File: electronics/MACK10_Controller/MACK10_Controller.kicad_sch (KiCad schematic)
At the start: 31 parts, among them J1 Stepper Motor, J10 I/O, J3 Load Cell, J4 24V IN, J5 SSD1306, J6 INPUT, J7 E_STOP, J8 LIM_TOP, J9 LIM_BOT, U1 U1 ESP32_DEVKIT_30P, U2 HX711, U3 TMC2208, U4 LM2596 Buck Converter

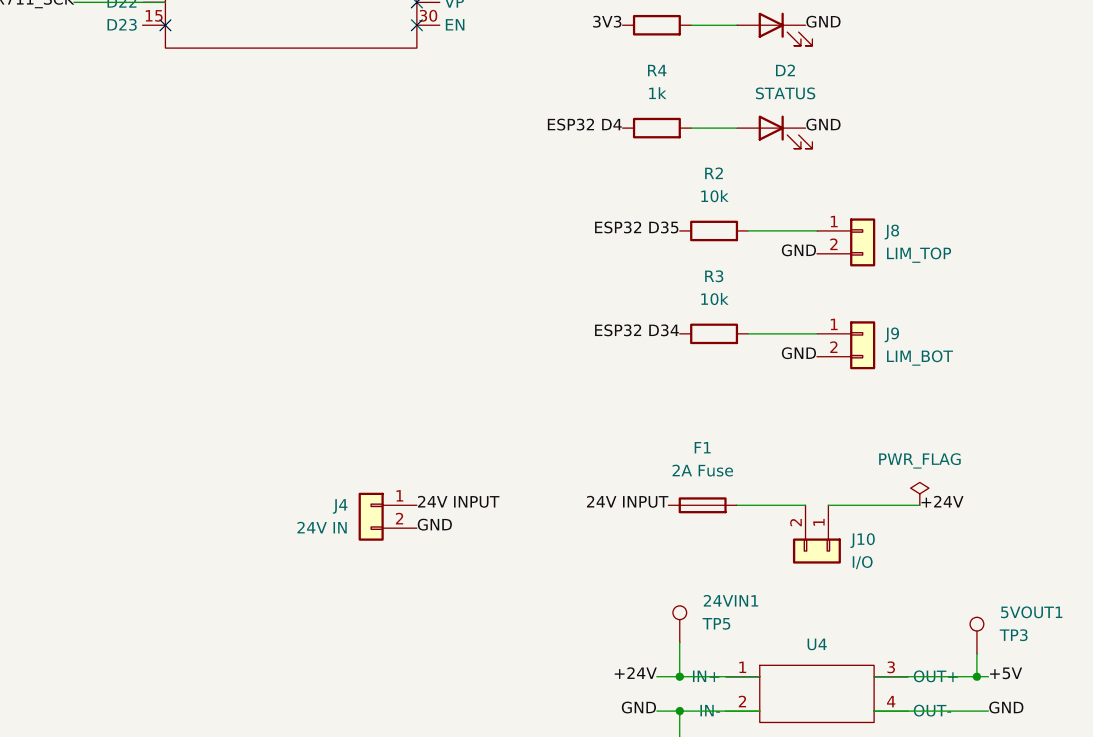
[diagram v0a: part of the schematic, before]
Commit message: Add Todo and various PCB updates
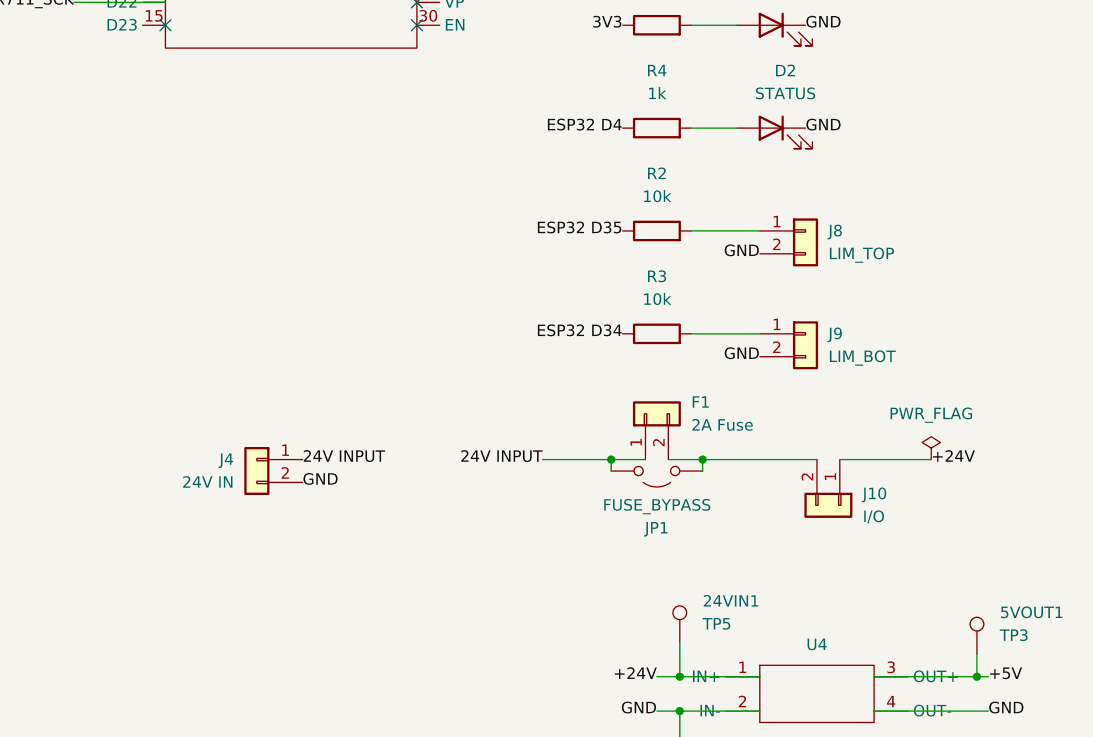
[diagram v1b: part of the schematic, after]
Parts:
- added JP1: FUSE_BYPASS, Jumper:SolderJumper-2_P1.3mm_Open_Pad1.0x1.5mm, symbol Jumper:Jumper_2_Open
- C1: footprint Capacitor_THT:CP_Radial_D8.0mm_P3.50mm -> Capacitor_SMD:CP_Elec_6.3x5.4
- C2: footprint Capacitor_THT:C_Disc_D5.0mm_W2.5mm_P5.00mm -> Capacitor_SMD:C_0603_1608Metric
- F1: footprint Fuse:Fuseholder_Blade_Mini_Keystone_3568 -> Connector_JST:JST_XH_B2B-XH-A_1x02_P2.50mm_Vertical; symbol Device:Fuse -> Connector_Generic:Conn_01x02
- J10: footprint Connector_PinHeader_2.54mm:PinHeader_1x02_P2.54mm_Vertical -> Connector_JST:JST_XH_B2B-XH-A_1x02_P2.50mm_Vertical
- R1, R2, R3, R4: footprint Resistor_THT:R_Axial_DIN0207_L6.3mm_D2.5mm_P10.16mm_Horizontal -> Resistor_SMD:R_0603_1608Metric
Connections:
- net 24V INPUT: now also JP1.1 (A)
- net at F1.2 (Pin_2), J10.2 (Pin_2): now also JP1.2 (B)
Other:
- moved on the sheet: J10, J4, J8, J9, R2, R3
